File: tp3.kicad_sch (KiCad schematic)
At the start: 0 parts

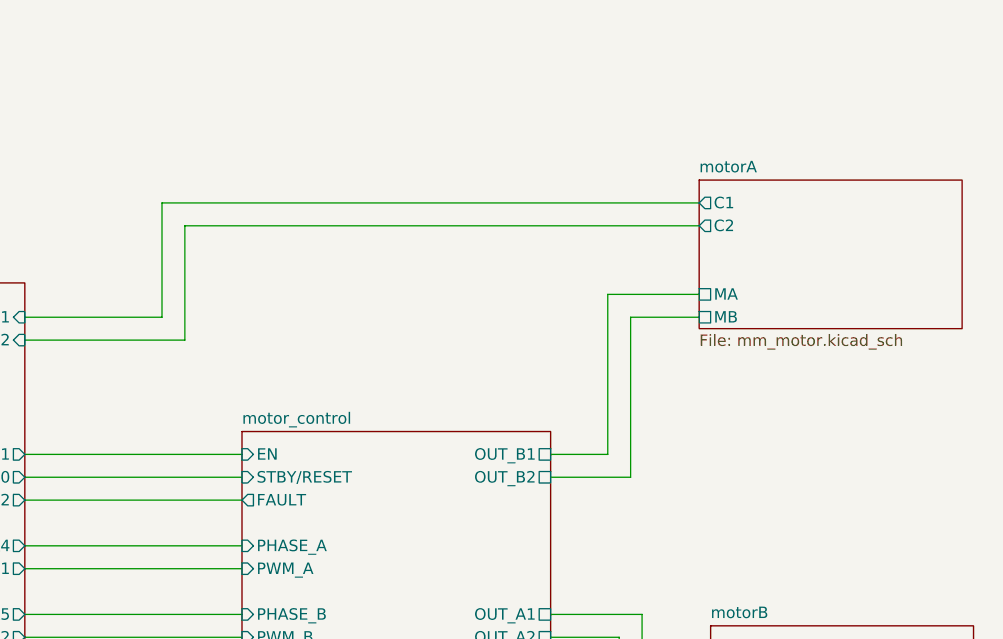
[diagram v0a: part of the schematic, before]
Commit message: tp5
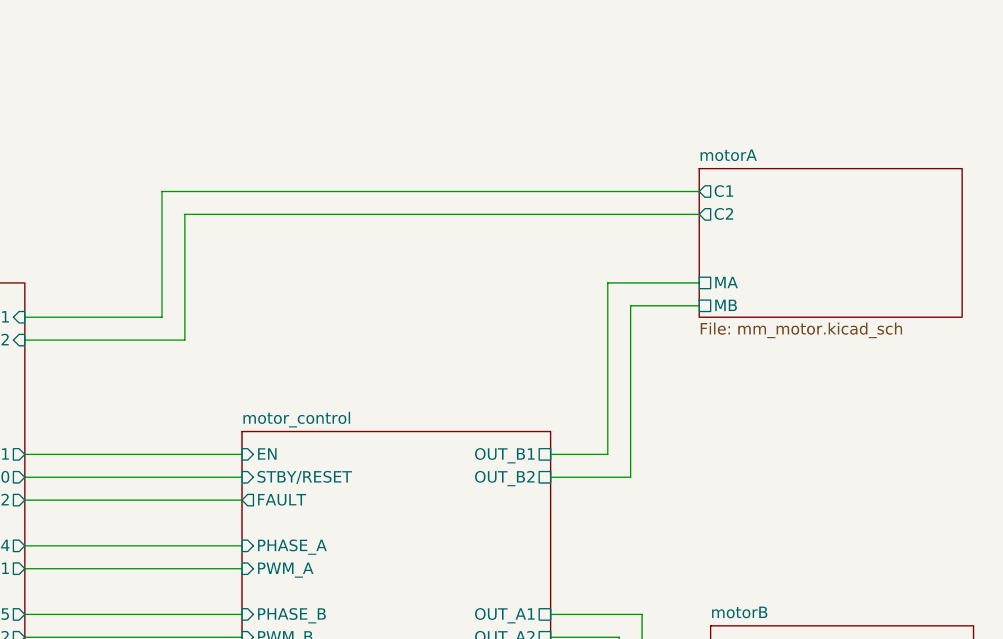
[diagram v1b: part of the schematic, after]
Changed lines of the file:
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@@
     (stroke (width 0) (type default))
   )
-  (wire (pts (xy 204.47 72.39) (xy 204.47 54.61))
+  (wire (pts (xy 204.47 72.39) (xy 204.47 53.34))
     (stroke (width 0) (type default))
   )
@@
     (stroke (width 0) (type default))
   )
-  (wire (pts (xy 157.48 46.99) (xy 157.48 59.69))
-    (stroke (width 0) (type default))
-  )
-  (wire (pts (xy 204.47 54.61) (xy 214.63 54.61))
+  (wire (pts (xy 157.48 45.72) (xy 157.48 59.69))
+    (stroke (width 0) (type default))
+  )
+  (wire (pts (xy 204.47 53.34) (xy 214.63 53.34))
     (stroke (width 0) (type default))
   )
@@
     (stroke (width 0) (type default))
   )
-  (wire (pts (xy 214.63 46.99) (xy 157.48 46.99))
-    (stroke (width 0) (type default))
-  )
-  (wire (pts (xy 207.01 57.15) (xy 214.63 57.15))
+  (wire (pts (xy 214.63 45.72) (xy 157.48 45.72))
+    (stroke (width 0) (type default))
+  )
+  (wire (pts (xy 207.01 55.88) (xy 214.63 55.88))
     (stroke (width 0) (type default))
   )
@@
     (stroke (width 0) (type default))
   )
-  (wire (pts (xy 154.94 57.15) (xy 154.94 44.45))
+  (wire (pts (xy 154.94 57.15) (xy 154.94 43.18))
     (stroke (width 0) (type default))
   )
@@
     (stroke (width 0) (type default))
   )
-  (wire (pts (xy 207.01 74.93) (xy 207.01 57.15))
+  (wire (pts (xy 207.01 74.93) (xy 207.01 55.88))
     (stroke (width 0) (type default))
   )
@@
     (stroke (width 0) (type default))
   )
-  (wire (pts (xy 154.94 44.45) (xy 214.63 44.45))
+  (wire (pts (xy 154.94 43.18) (xy 214.63 43.18))
     (stroke (width 0) (type default))
   )
@@
     )
     (instances
-      (project "tp2"
+      (project "tp3"
         (path "/d8fa4cba-2469-4231-847f-065b6b829f44" (page "4"))
       )
@@
     )
     (instances
-      (project "tp2"
+      (project "tp3"
         (path "/d8fa4cba-2469-4231-847f-065b6b829f44" (page "8"))
       )
@@
     )
     (instances
-      (project "tp2"
+      (project "tp3"
         (path "/d8fa4cba-2469-4231-847f-065b6b829f44" (page "6"))
       )
@@
     )
     (instances
-      (project "tp2"
+      (project "tp3"
         (path "/d8fa4cba-2469-4231-847f-065b6b829f44" (page "2"))
       )
     )
   )
-  (sheet (at 214.63 41.91) (size 29.21 16.51) (fields_autoplaced)
-    (stroke (width 0.1524) (type solid))
-    (fill (color 0 0 0 0.0000))
-    (property "Sheetname" "motorA" (at 214.63 41.1984 0)
-      (effects (font (size 1.27 1.27)) (justify left bottom))
-    )
-    (property "Sheetfile" "mm_motor.kicad_sch" (at 214.63 59.0046 0)
-      (effects (font (size 1.27 1.27)) (justify left top))
-    )
-    (pin "C1" output (at 214.63 44.45 180)
-      (effects (font (size 1.27 1.27)) (justify left))
-    )
-    (pin "MB" passive (at 214.63 57.15 180)
-      (effects (font (size 1.27 1.27)) (justify left))
-    )
-    (pin "C2" output (at 214.63 46.99 180)
-      (effects (font (size 1.27 1.27)) (justify left))
-    )
-    (pin "MA" passive (at 214.63 54.61 180)
-      (effects (font (size 1.27 1.27)) (justify left))
-    )
-    (instances
-      (project "tp2"
+  (sheet (at 214.63 40.64) (size 29.21 16.51) (fields_autoplaced)
+    (stroke (width 0.1524) (type solid))
+    (fill (color 0 0 0 0.0000))
+    (property "Sheetname" "motorA" (at 214.63 39.9284 0)
+      (effects (font (size 1.27 1.27)) (justify left bottom))
+    )
+    (property "Sheetfile" "mm_motor.kicad_sch" (at 214.63 57.7346 0)
+      (effects (font (size 1.27 1.27)) (justify left top))
+    )
+    (pin "C1" output (at 214.63 43.18 180)
+      (effects (font (size 1.27 1.27)) (justify left))
+    )
+    (pin "MB" passive (at 214.63 55.88 180)
+      (effects (font (size 1.27 1.27)) (justify left))
+    )
+    (pin "C2" output (at 214.63 45.72 180)
+      (effects (font (size 1.27 1.27)) (justify left))
+    )
+    (pin "MA" passive (at 214.63 53.34 180)
+      (effects (font (size 1.27 1.27)) (justify left))
+    )
+    (instances
+      (project "tp3"
         (path "/d8fa4cba-2469-4231-847f-065b6b829f44" (page "5"))
       )
@@
     )
     (instances
-      (project "tp2"
+      (project "tp3"
         (path "/d8fa4cba-2469-4231-847f-065b6b829f44" (page "3"))
       )
@@
     )
     (instances
-      (project "tp2"
+      (project "tp3"
         (path "/d8fa4cba-2469-4231-847f-065b6b829f44" (page "7"))
       )
